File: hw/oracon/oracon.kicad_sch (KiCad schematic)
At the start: 108 parts, among them J2 SIM_Card, J3 USB_A, J4 Conn_Coaxial, J5 USB_C_Receptacle_USB2.0_16P, Q1 SS8050, Q2 SS8050, Q3 SS8050, Q5 SS8050, SW1 SW_Push, U1 TP5100, U2 AMS1117-3.3, U3 ESP32-S3-MINI-1U, U4 CH343P, U5 TPS61022, U6 MAX3232, U7 SIM7022

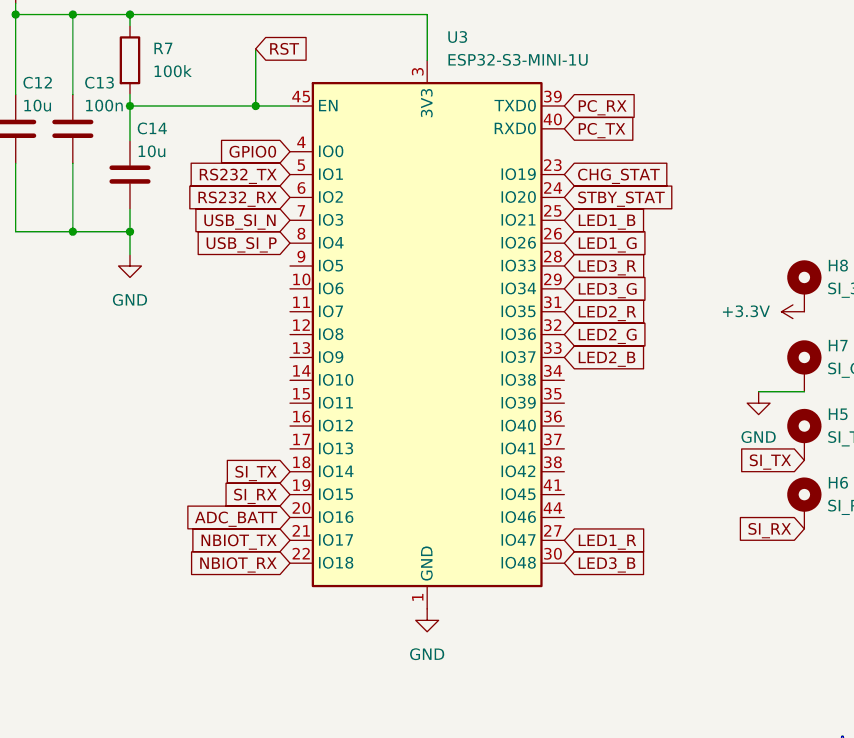
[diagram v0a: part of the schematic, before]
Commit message: Further routing
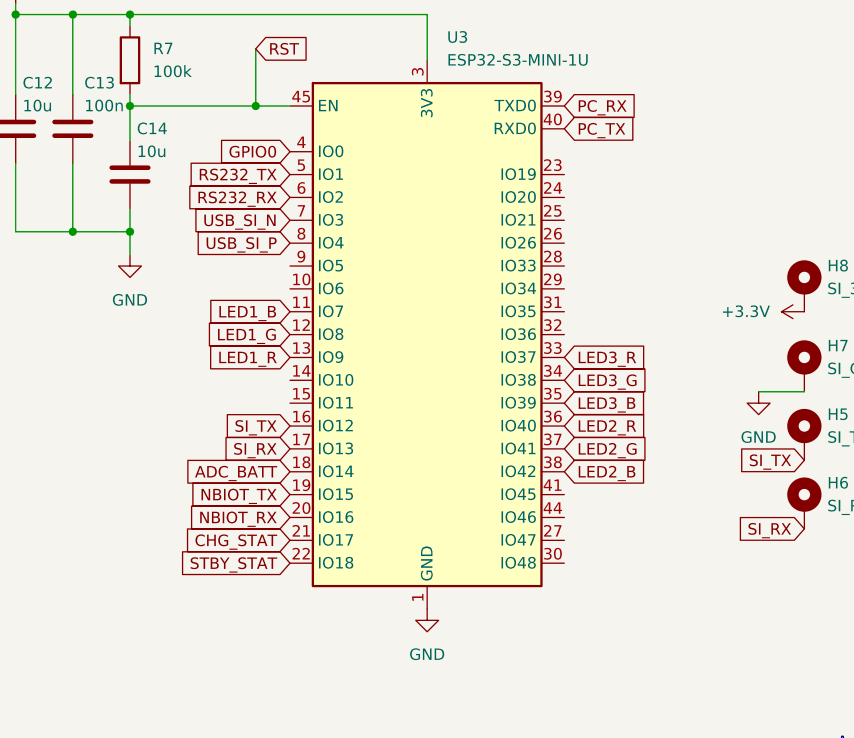
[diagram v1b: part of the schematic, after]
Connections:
- net ADC_BATT: now also U3.18 (IO14); no longer U3.20 (IO16)
- net CHG_STAT: now also U3.21 (IO17); no longer U3.23 (IO19)
- net LED1_B: now also U3.11 (IO7); no longer U3.25 (IO21)
- net LED1_G: now also U3.12 (IO8); no longer U3.26 (IO26)
- net LED1_R: now also U3.13 (IO9); no longer U3.27 (IO47)
- net LED2_B: now also U3.38 (IO42); no longer U3.33 (IO37)
- net LED2_G: now also U3.37 (IO41); no longer U3.32 (IO36)
- net LED2_R: now also U3.36 (IO40); no longer U3.31 (IO35)
- net LED3_B: now also U3.35 (IO39); no longer U3.30 (IO48)
- net LED3_G: now also U3.34 (IO38); no longer U3.29 (IO34)
- net LED3_R: now also U3.33 (IO37); no longer U3.28 (IO33)
- net NBIOT_RX: now also U3.20 (IO16); no longer U3.22 (IO18)
- net NBIOT_TX: now also U3.19 (IO15); no longer U3.21 (IO17)
- net SI_RX: now also U3.17 (IO13); no longer U3.19 (IO15)
- net SI_TX: now also U3.16 (IO12); no longer U3.18 (IO14)
- net STBY_STAT: now also U3.22 (IO18); no longer U3.24 (IO20)
